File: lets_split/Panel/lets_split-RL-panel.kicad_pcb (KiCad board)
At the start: 2 copper layers, 229 x 78 mm, 116 parts, among them J2 CONN_01X04, SW1 SW_PUSH, SW10 SW_PUSH, SW11 SW_PUSH, SW12 SW_PUSH, SW13 SW_PUSH, SW14 SW_PUSH, SW15 SW_PUSH, SW16 SW_PUSH, SW17 SW_PUSH, SW18 SW_PUSH, SW19 SW_PUSH, SW2 SW_PUSH, SW20 SW_PUSH, SW21 SW_PUSH, SW22 SW_PUSH, SW23 SW_PUSH, SW24 SW_PUSH, SW3 SW_PUSH, SW4 SW_PUSH, SW5 SW_PUSH, SW6 SW_PUSH, SW7 SW_PUSH, SW8 SW_PUSH, SW9 SW_PUSH, U1 ArduinoProMicro

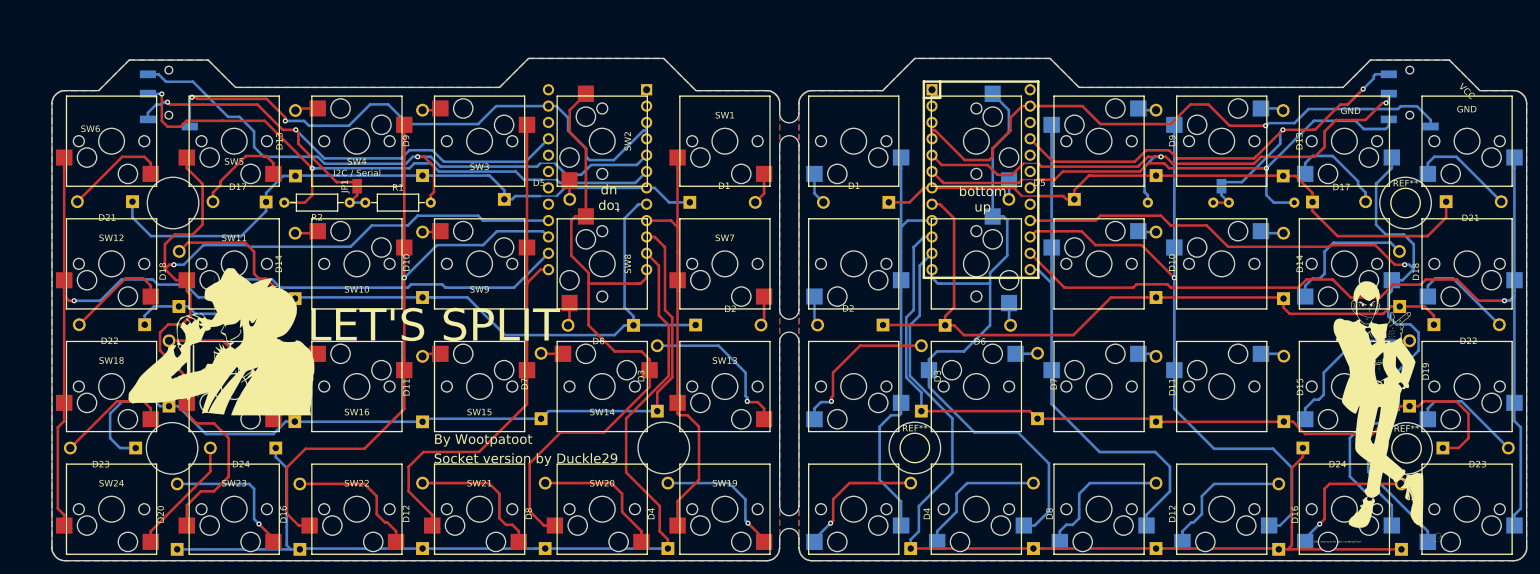
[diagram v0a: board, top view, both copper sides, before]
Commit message: Finished and panelized V3
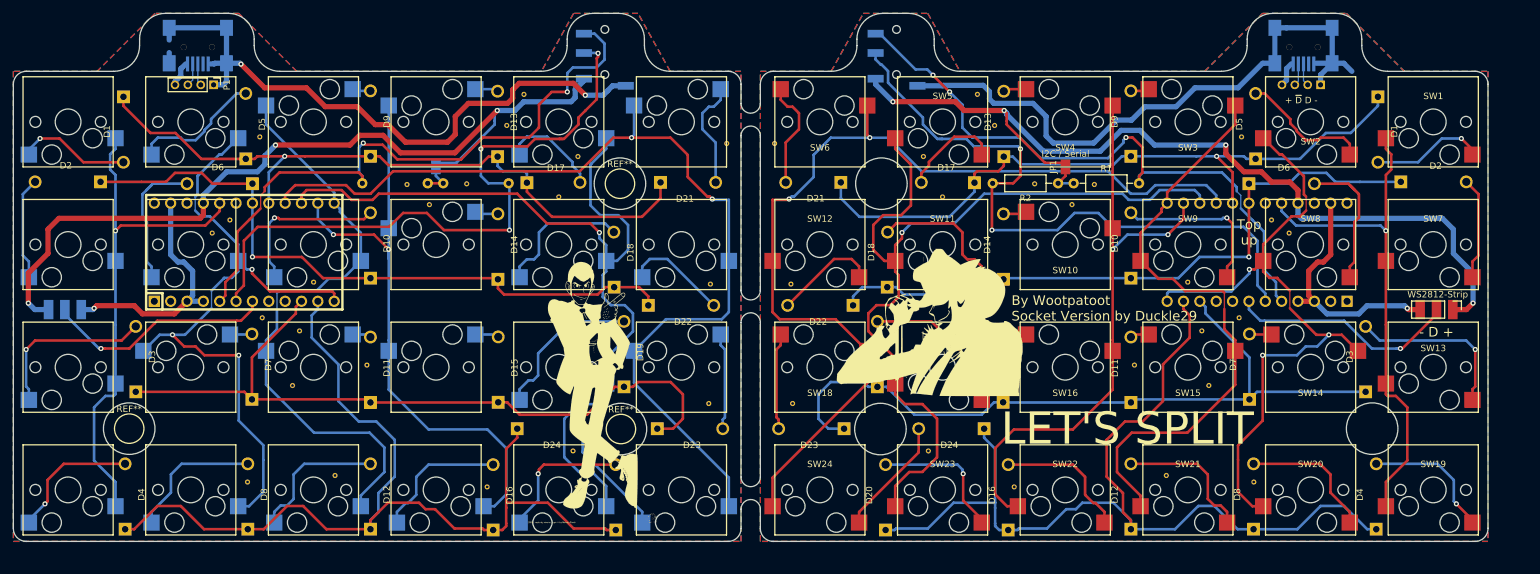
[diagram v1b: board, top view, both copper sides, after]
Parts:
- removed the D1 at (163.9, 81.3)
- removed the D1 at (133.1, 81.3)
- removed the D10 at (205.5, 96.1)
- removed the D10 at (91.5, 96.1)
- removed the D11 at (205.5, 115.4)
- removed the D11 at (91.5, 115.4)
- removed the D12 at (205.5, 135.1)
- removed the D12 at (91.5, 135.1)
- removed the D13 at (225.2, 77.2)
- removed the D13 at (71.8, 77.2)
- removed the D14 at (225.2, 96.3)
- removed the D14 at (71.8, 96.3)
- removed the D15 at (225.3, 115.4)
- removed the D15 at (71.7, 115.4)
- removed the D16 at (224.5, 135.2)
- removed the D16 at (72.5, 135.2)
- removed the D17 at (229.8, 81.3)
- removed the D17 at (67.2, 81.3)
- removed the D18 at (243.3, 97.5)
- removed the D18 at (53.7, 97.5)
- removed the D19 at (244.8, 113.0)
- removed the D19 at (52.2, 113.0)
- removed the D2 at (163.1, 100.4)
- removed the D2 at (133.9, 100.4)
- removed the D20 at (243.6, 135.2)
- removed the D20 at (53.4, 135.2)
- removed the D21 at (248.9, 81.2)
- removed the D21 at (48.1, 81.2)
- removed the D22 at (248.6, 100.3)
- removed the D22 at (48.4, 100.3)
- removed the D23 at (250.0, 119.5)
- removed the D23 at (47.0, 119.5)
- removed the D24 at (228.2, 119.5)
- removed the D24 at (68.8, 119.5)
- removed the D3 at (169.0, 113.8)
- removed the D3 at (128.0, 113.8)
- removed the D4 at (167.4, 135.1)
- removed the D4 at (129.6, 135.1)
- removed the D5 at (192.8, 80.9)
- removed the D5 at (104.2, 80.9)
- removed the D6 at (172.7, 100.5)
- removed the D6 at (124.3, 100.5)
- removed the D7 at (187.1, 115.0)
- removed the D7 at (110.0, 115.0)
- removed the D8 at (186.4, 135.1)
- removed the D8 at (110.6, 135.1)
- removed the D9 at (205.5, 77.2)
- removed the D9 at (91.5, 77.2)
- removed the G*** at (240.0, 112.8)
- removed the G*** at (231.8, 103.0)
- removed the G*** at (65.2, 103.0)
- removed the G*** at (57.0, 112.8)
- removed the J2 at (244.9, 64.3)
- removed the J2 at (52.1, 64.3)
- removed the JP1 at (215.6, 78.8)
- removed the JP1 at (81.4, 78.8)
- removed the R1 at (214.3, 81.4)
- removed the R1 at (82.7, 81.4)
- removed the R2 at (216.8, 81.4)
- removed the R2 at (80.2, 81.4)
- removed the REF** at (168.0, 119.5)
- removed the REF** at (244.3, 119.5)
- removed the REF** at (244.2, 81.5)
- removed the REF** at (52.8, 81.5)
- removed the REF** at (52.6, 119.5)
- removed the REF** at (129.0, 119.5)
- removed the SW1 at (158.5, 71.8)
- removed the SW1 at (138.5, 71.8)
- removed the SW10 at (215.7, 90.9)
- removed the SW10 at (81.3, 90.9)
- removed the SW11 at (234.7, 90.9)
- removed the SW11 at (62.3, 90.9)
- removed the SW12 at (253.8, 90.9)
- removed the SW12 at (43.2, 90.9)
- removed the SW13 at (158.5, 110.0)
- removed the SW13 at (138.5, 110.0)
- removed the SW14 at (177.6, 110.0)
- removed the SW14 at (119.5, 110.0)
- removed the SW15 at (196.6, 110.0)
- removed the SW15 at (100.4, 110.0)
- removed the SW16 at (215.7, 110.0)
- removed the SW16 at (81.3, 110.0)
- removed the SW17 at (234.7, 110.0)
- removed the SW17 at (62.3, 110.0)
- removed the SW18 at (253.8, 110.0)
- removed the SW18 at (43.2, 110.0)
- removed the SW19 at (158.5, 129.0)
- removed the SW19 at (138.5, 129.0)
- removed the SW2 at (177.6, 71.8)
- removed the SW2 at (119.5, 71.8)
- removed the SW20 at (177.6, 129.0)
- removed the SW20 at (119.5, 129.0)
- removed the SW21 at (196.6, 129.0)
- removed the SW21 at (100.4, 129.0)
- removed the SW22 at (215.7, 129.0)
- removed the SW22 at (81.3, 129.0)
- removed the SW23 at (234.7, 129.0)
- removed the SW23 at (62.3, 129.0)
- removed the SW24 at (253.8, 129.0)
- removed the SW24 at (43.2, 129.0)
- removed the SW3 at (196.6, 71.8)
- removed the SW3 at (100.4, 71.8)
- removed the SW4 at (215.7, 71.8)
- removed the SW4 at (81.3, 71.8)
- removed the SW5 at (234.7, 71.8)
- removed the SW5 at (62.3, 71.8)
- removed the SW6 at (253.8, 71.8)
- removed the SW6 at (43.2, 71.8)
- removed the SW7 at (158.5, 90.9)
- removed the SW7 at (138.5, 90.9)
- removed the SW8 at (177.6, 90.9)
- removed the SW8 at (119.5, 90.9)
- removed the SW9 at (196.6, 90.9)
- removed the SW9 at (100.4, 90.9)
- removed the U1 at (178.3, 77.8)
- removed the U1 at (118.7, 77.8)
- added D1: D, Diodes_ThroughHole:Diode_DO-41_SOD81_Horizontal_RM10, B.Cu at (239.9, 65.0)
- added D1: D, Diodes_ThroughHole:Diode_DO-41_SOD81_Horizontal_RM10, F.Cu at (45.1, 65.0)
- added D10: D, Diodes_ThroughHole:Diode_DO-41_SOD81_Horizontal_RM10, B.Cu at (201.5, 93.1)
- added D10: D, Diodes_ThroughHole:Diode_DO-41_SOD81_Horizontal_RM10, F.Cu at (83.5, 93.1)
- added D11: D, Diodes_ThroughHole:Diode_DO-41_SOD81_Horizontal_RM10, B.Cu at (201.5, 112.4)
- added D11: D, Diodes_ThroughHole:Diode_DO-41_SOD81_Horizontal_RM10, F.Cu at (83.5, 112.4)
- added D12: D, Diodes_ThroughHole:Diode_DO-41_SOD81_Horizontal_RM10, B.Cu at (201.5, 132.1)
- added D12: D, Diodes_ThroughHole:Diode_DO-41_SOD81_Horizontal_RM10, F.Cu at (83.5, 132.1)
- added D13: D, Diodes_ThroughHole:Diode_DO-41_SOD81_Horizontal_RM10, B.Cu at (181.8, 74.2)
- added D13: D, Diodes_ThroughHole:Diode_DO-41_SOD81_Horizontal_RM10, F.Cu at (103.2, 74.2)
- added D14: D, Diodes_ThroughHole:Diode_DO-41_SOD81_Horizontal_RM10, B.Cu at (181.8, 93.3)
- added D14: D, Diodes_ThroughHole:Diode_DO-41_SOD81_Horizontal_RM10, F.Cu at (103.2, 93.3)
- added D15: D, Diodes_ThroughHole:Diode_DO-41_SOD81_Horizontal_RM10, B.Cu at (181.7, 112.4)
- added D15: D, Diodes_ThroughHole:Diode_DO-41_SOD81_Horizontal_RM10, F.Cu at (103.3, 112.4)
- added D16: D, Diodes_ThroughHole:Diode_DO-41_SOD81_Horizontal_RM10, B.Cu at (182.5, 132.2)
- added D16: D, Diodes_ThroughHole:Diode_DO-41_SOD81_Horizontal_RM10, F.Cu at (102.5, 132.2)
- added D17: D, Diodes_ThroughHole:Diode_DO-41_SOD81_Horizontal_RM10, B.Cu at (177.2, 78.3)
- added D17: D, Diodes_ThroughHole:Diode_DO-41_SOD81_Horizontal_RM10, F.Cu at (107.8, 78.3)
- added D18: D, Diodes_ThroughHole:Diode_DO-41_SOD81_Horizontal_RM10, B.Cu at (163.7, 94.5)
- added D18: D, Diodes_ThroughHole:Diode_DO-41_SOD81_Horizontal_RM10, F.Cu at (121.3, 94.5)
- added D19: D, Diodes_ThroughHole:Diode_DO-41_SOD81_Horizontal_RM10, B.Cu at (162.2, 110.0)
- added D19: D, Diodes_ThroughHole:Diode_DO-41_SOD81_Horizontal_RM10, F.Cu at (122.8, 110.0)
- added D2: D, Diodes_ThroughHole:Diode_DO-41_SOD81_Horizontal_RM10, B.Cu at (243.5, 78.2)
- added D2: D, Diodes_ThroughHole:Diode_DO-41_SOD81_Horizontal_RM10, F.Cu at (41.5, 78.2)
- added D20: D, Diodes_ThroughHole:Diode_DO-41_SOD81_Horizontal_RM10, B.Cu at (163.4, 132.2)
- added D20: D, Diodes_ThroughHole:Diode_DO-41_SOD81_Horizontal_RM10, F.Cu at (121.6, 132.2)
- added D21: D, Diodes_ThroughHole:Diode_DO-41_SOD81_Horizontal_RM10, B.Cu at (158.1, 78.2)
- added D21: D, Diodes_ThroughHole:Diode_DO-41_SOD81_Horizontal_RM10, F.Cu at (126.9, 78.2)
- added D22: D, Diodes_ThroughHole:Diode_DO-41_SOD81_Horizontal_RM10, B.Cu at (158.4, 97.3)
- added D22: D, Diodes_ThroughHole:Diode_DO-41_SOD81_Horizontal_RM10, F.Cu at (126.6, 97.3)
- added D23: D, Diodes_ThroughHole:Diode_DO-41_SOD81_Horizontal_RM10, B.Cu at (157.0, 116.5)
- added D23: D, Diodes_ThroughHole:Diode_DO-41_SOD81_Horizontal_RM10, F.Cu at (128.0, 116.5)
- added D24: D, Diodes_ThroughHole:Diode_DO-41_SOD81_Horizontal_RM10, B.Cu at (178.8, 116.5)
- added D24: D, Diodes_ThroughHole:Diode_DO-41_SOD81_Horizontal_RM10, F.Cu at (106.2, 116.5)
- added D3: D, Diodes_ThroughHole:Diode_DO-41_SOD81_Horizontal_RM10, B.Cu at (238.0, 110.8)
- added D3: D, Diodes_ThroughHole:Diode_DO-41_SOD81_Horizontal_RM10, F.Cu at (47.0, 110.8)
- added D4: D, Diodes_ThroughHole:Diode_DO-41_SOD81_Horizontal_RM10, B.Cu at (239.6, 132.1)
- added D4: D, Diodes_ThroughHole:Diode_DO-41_SOD81_Horizontal_RM10, F.Cu at (45.4, 132.1)
- added D5: D, Diodes_ThroughHole:Diode_DO-41_SOD81_Horizontal_RM10, B.Cu at (220.9, 74.6)
- added D5: D, Diodes_ThroughHole:Diode_DO-41_SOD81_Horizontal_RM10, F.Cu at (64.1, 74.6)
- added D6: D, Diodes_ThroughHole:Diode_DO-41_SOD81_Horizontal_RM10, B.Cu at (219.9, 78.4)
- added D6: D, Diodes_ThroughHole:Diode_DO-41_SOD81_Horizontal_RM10, F.Cu at (65.1, 78.4)
- added D7: D, Diodes_ThroughHole:Diode_DO-41_SOD81_Horizontal_RM10, B.Cu at (219.9, 112.0)
- added D7: D, Diodes_ThroughHole:Diode_DO-41_SOD81_Horizontal_RM10, F.Cu at (65.0, 112.0)
- added D8: D, Diodes_ThroughHole:Diode_DO-41_SOD81_Horizontal_RM10, B.Cu at (220.6, 132.1)
- added D8: D, Diodes_ThroughHole:Diode_DO-41_SOD81_Horizontal_RM10, F.Cu at (64.4, 132.1)
- added D9: D, Diodes_ThroughHole:Diode_DO-41_SOD81_Horizontal_RM10, B.Cu at (201.5, 74.2)
- added D9: D, Diodes_ThroughHole:Diode_DO-41_SOD81_Horizontal_RM10, F.Cu at (83.5, 74.2)
- added G***: LOGO, LOGO, B.Cu at (167.0, 109.8)
- added G***: LOGO, LOGO, F.Cu at (175.2, 100.0)
- added G***: LOGO, LOGO, B.Cu at (109.8, 100.0)
- added G***: LOGO, LOGO, F.Cu at (118.0, 109.8)
- added J2: CONN_01X04, Connectors:4ucon-20153, B.Cu at (165.1, 58.0)
- added J2: CONN_01X04, Connectors:4ucon-20153, B.Cu at (119.9, 58.0)
- added JP1: I2C / Serial, Jumpers:Solder-jumper-NO, F.Cu at (191.4, 75.8)
- added JP1: I2C / Serial, Jumpers:Solder-jumper-NO, B.Cu at (93.6, 75.8)
- added P1: USB-rewire, Pin_Headers:Pin_Header_Straight_1x04_Pitch2.00mm, B.Cu at (231.0, 63.1)
- added P1: USB-rewire, Pin_Headers:Pin_Header_Straight_1x04_Pitch2.00mm, F.Cu at (59.1, 63.1)
- added P2: USB_OTG, Connectors:USB-Mini-B-SMD, B.Cu at (228.3, 56.0)
- added P2: USB_OTG, Connectors:USB-Mini-B-SMD, B.Cu at (56.6, 56.0)
- added P3: WS2812-Strip, SMD_PAD_1x03_Pitch2.54mm, F.Cu at (251.5, 98.0)
- added P3: WS2812-Strip, SMD_PAD_1x03_Pitch2.54mm, B.Cu at (33.5, 98.0)
- added R1: 4k7, Resistors_ThroughHole:R_Axial_DIN0207_L6.3mm_D2.5mm_P10.16mm_Horizontal, F.Cu at (192.7, 78.4)
- added R1: 4k7, Resistors_ThroughHole:R_Axial_DIN0207_L6.3mm_D2.5mm_P10.16mm_Horizontal, B.Cu at (92.3, 78.4)
- added R2: 4k7, Resistors_ThroughHole:R_Axial_DIN0207_L6.3mm_D2.5mm_P10.16mm_Horizontal, F.Cu at (190.2, 78.4)
- added R2: 4k7, Resistors_ThroughHole:R_Axial_DIN0207_L6.3mm_D2.5mm_P10.16mm_Horizontal, B.Cu at (94.8, 78.4)
- added REF**: 1pin, Connect:1pin, B.Cu at (239.0, 116.5)
- added REF**: 1pin, Connect:1pin, B.Cu at (170.1, 120.0)
- added REF**: 1pin, Connect:1pin, B.Cu at (149.0, 112.6)
- added REF**: 1pin, Connect:1pin, B.Cu at (148.8, 94.0)
- added REF**: 1pin, Connect:1pin, B.Cu at (146.2, 72.2)
- added REF**: 1pin, Connect:1pin, B.Cu at (180.4, 69.4)
- added REF**: 1pin, Connect:1pin, B.Cu at (169.3, 74.2)
- added REF**: 1pin, Connect:1pin, B.Cu at (218.7, 71.2)
- added REF**: 1pin, Connect:1pin, B.Cu at (212.6, 101.3)
- added REF**: 1pin, Connect:1pin, B.Cu at (218.3, 99.3)
- added REF**: 1pin, Connect:1pin, B.Cu at (226.1, 86.1)
- added REF**: 1pin, Connect:1pin, B.Cu at (162.7, 116.5)
- added REF**: 1pin, Connect:1pin, B.Cu at (223.4, 84.1)
- added REF**: 1pin, Connect:1pin, B.Cu at (210.4, 93.7)
- added REF**: 1pin, Connect:1pin, B.Cu at (172.3, 80.5)
- added REF**: 1pin, Connect:1pin, B.Cu at (192.4, 81.7)
- added REF**: 1pin, Connect:1pin, B.Cu at (195.9, 78.6)
- added REF**: 1pin, Connect:1pin, B.Cu at (186.6, 78.5)
- added REF**: 1pin, Connect:1pin, F.Cu at (98.4, 78.5)
- added REF**: 1pin, Connect:1pin, F.Cu at (89.1, 78.6)
- added REF**: 1pin, Connect:1pin, F.Cu at (92.6, 81.7)
- added REF**: 1pin, Connect:1pin, F.Cu at (112.7, 80.5)
- added REF**: 1pin, Connect:1pin, B.Cu at (162.8, 78.5)
- added REF**: 1pin, Connect:1pin, F.Cu at (74.6, 93.7)
- added REF**: 1pin, Connect:1pin, F.Cu at (61.6, 84.1)
- added REF**: 1pin, Connect:1pin, F.Cu at (58.9, 86.1)
- added REF**: 1pin, Connect:1pin, F.Cu at (66.7, 99.3)
- added REF**: 1pin, Connect:1pin, F.Cu at (72.4, 101.3)
- added REF**: 1pin, Connect:1pin, F.Cu at (66.3, 71.2)
- added REF**: 1pin, Connect:1pin, F.Cu at (115.7, 74.2)
- added REF**: 1pin, Connect:1pin, F.Cu at (104.6, 69.4)
- added REF**: 1pin, Connect:1pin, F.Cu at (138.8, 72.2)
- added REF**: 1pin, Connect:1pin, F.Cu at (136.2, 94.0)
- added REF**: 1pin, Connect:1pin, B.Cu at (177.7, 64.6)
- added REF**: 1pin, Connect:1pin, F.Cu at (136.0, 112.6)
- added REF**: 1pin, Connect:1pin, F.Cu at (114.9, 120.0)
- added REF**: 1pin, Connect:1pin, F.Cu at (101.6, 125.5)
- added REF**: 1pin, Connect:1pin, F.Cu at (64.4, 124.8)
- added REF**: 1pin, Connect:1pin, F.Cu at (78.0, 123.8)
- added REF**: 1pin, Connect:1pin, F.Cu at (71.3, 109.8)
- added REF**: 1pin, Connect:1pin, F.Cu at (82.9, 106.6)
- added REF**: 1pin, Connect:1pin, F.Cu at (107.3, 64.6)
- added REF**: 1pin, Connect:1pin, F.Cu at (122.2, 78.5)
- added REF**: 1pin, Connect:1pin, F.Cu at (122.3, 116.5)
- added REF**: 1pin, Connect:1pin, B.Cu at (202.1, 106.6)
- added REF**: 1pin, Connect:1pin, F.Cu at (46.0, 116.5)
- added REF**: 1pin, Connect:1pin, B.Cu at (213.7, 109.8)
- added REF**: 1pin, Connect:1pin, B.Cu at (207.0, 123.8)
- added REF**: 1pin, Connect:1pin, B.Cu at (220.6, 124.8)
- added REF**: 1pin, Connect:1pin, B.Cu at (183.4, 125.5)
- added SW1: SW_PUSH, CherryMX:Kailh-socket, B.Cu at (248.5, 68.8)
- added SW1: SW_PUSH, CherryMX:Kailh-socket, F.Cu at (36.5, 68.8)
- added SW10: SW_PUSH, CherryMX:Kailh-socket, B.Cu at (191.3, 87.9)
- added SW10: SW_PUSH, CherryMX:Kailh-socket, F.Cu at (93.7, 87.9)
- added SW11: SW_PUSH, CherryMX:Kailh-socket, B.Cu at (172.3, 87.9)
- added SW11: SW_PUSH, CherryMX:Kailh-socket, F.Cu at (112.7, 87.9)
- added SW12: SW_PUSH, CherryMX:Kailh-socket, B.Cu at (153.2, 87.9)
- added SW12: SW_PUSH, CherryMX:Kailh-socket, F.Cu at (131.8, 87.9)
- added SW13: SW_PUSH, CherryMX:Kailh-socket, B.Cu at (248.5, 107.0)
- added SW13: SW_PUSH, CherryMX:Kailh-socket, F.Cu at (36.5, 107.0)
- added SW14: SW_PUSH, CherryMX:Kailh-socket, B.Cu at (229.4, 107.0)
- added SW14: SW_PUSH, CherryMX:Kailh-socket, F.Cu at (55.5, 107.0)
- added SW15: SW_PUSH, CherryMX:Kailh-socket, B.Cu at (210.4, 107.0)
- added SW15: SW_PUSH, CherryMX:Kailh-socket, F.Cu at (74.6, 107.0)
- added SW16: SW_PUSH, CherryMX:Kailh-socket, B.Cu at (191.3, 107.0)
- added SW16: SW_PUSH, CherryMX:Kailh-socket, F.Cu at (93.7, 107.0)
- added SW17: SW_PUSH, CherryMX:Kailh-socket, B.Cu at (172.3, 107.0)
- added SW17: SW_PUSH, CherryMX:Kailh-socket, F.Cu at (112.7, 107.0)
- added SW18: SW_PUSH, CherryMX:Kailh-socket, B.Cu at (153.2, 107.0)
- added SW18: SW_PUSH, CherryMX:Kailh-socket, F.Cu at (131.8, 107.0)
- added SW19: SW_PUSH, CherryMX:Kailh-socket, B.Cu at (248.5, 126.0)
- added SW19: SW_PUSH, CherryMX:Kailh-socket, F.Cu at (36.5, 126.0)
- added SW2: SW_PUSH, CherryMX:Kailh-socket, B.Cu at (229.4, 68.8)
- added SW2: SW_PUSH, CherryMX:Kailh-socket, F.Cu at (55.5, 68.8)
- added SW20: SW_PUSH, CherryMX:Kailh-socket, B.Cu at (229.4, 126.0)
- added SW20: SW_PUSH, CherryMX:Kailh-socket, F.Cu at (55.5, 126.0)
- added SW21: SW_PUSH, CherryMX:Kailh-socket, B.Cu at (210.4, 126.0)
- added SW21: SW_PUSH, CherryMX:Kailh-socket, F.Cu at (74.6, 126.0)
- added SW22: SW_PUSH, CherryMX:Kailh-socket, B.Cu at (191.3, 126.0)
- added SW22: SW_PUSH, CherryMX:Kailh-socket, F.Cu at (93.7, 126.0)
- added SW23: SW_PUSH, CherryMX:Kailh-socket, B.Cu at (172.3, 126.0)
- added SW23: SW_PUSH, CherryMX:Kailh-socket, F.Cu at (112.7, 126.0)
- added SW24: SW_PUSH, CherryMX:Kailh-socket, B.Cu at (153.2, 126.0)
- added SW24: SW_PUSH, CherryMX:Kailh-socket, F.Cu at (131.8, 126.0)
- added SW3: SW_PUSH, CherryMX:Kailh-socket, B.Cu at (210.4, 68.8)
- added SW3: SW_PUSH, CherryMX:Kailh-socket, F.Cu at (74.6, 68.8)
- added SW4: SW_PUSH, CherryMX:Kailh-socket, B.Cu at (191.3, 68.8)
- added SW4: SW_PUSH, CherryMX:Kailh-socket, F.Cu at (93.7, 68.8)
- added SW5: SW_PUSH, CherryMX:Kailh-socket, B.Cu at (172.3, 68.8)
- added SW5: SW_PUSH, CherryMX:Kailh-socket, F.Cu at (112.7, 68.8)
- added SW6: SW_PUSH, Kailh-socket, B.Cu at (153.2, 68.8)
- added SW6: SW_PUSH, Kailh-socket, F.Cu at (131.8, 68.8)
- added SW7: SW_PUSH, CherryMX:Kailh-socket, B.Cu at (248.5, 87.9)
- added SW7: SW_PUSH, CherryMX:Kailh-socket, F.Cu at (36.5, 87.9)
- added SW8: SW_PUSH, CherryMX:Kailh-socket, B.Cu at (229.4, 87.9)
- added SW8: SW_PUSH, CherryMX:Kailh-socket, F.Cu at (55.5, 87.9)
- added SW9: SW_PUSH, CherryMX:Kailh-socket, B.Cu at (210.4, 87.9)
- added SW9: SW_PUSH, CherryMX:Kailh-socket, F.Cu at (74.6, 87.9)
- added U1: ArduinoProMicro, plug-in-modules:ArduinoProMicro, B.Cu at (221.1, 89.1)
- added U1: ArduinoProMicro, plug-in-modules:ArduinoProMicro, F.Cu at (63.9, 89.1)
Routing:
- net VCC: track 162.2 -> 264.9 mm, vias 4 -> 7
- net GND: track 187.7 -> 274.0 mm, vias 3 -> 4
- net Net-(P3-Pad2): track 0.00 -> 71.7 mm, vias 0 -> 2
- net Net-(D10-Pad2): track 5.64 -> 50.6 mm, vias 0 -> 2
- net Net-(D6-Pad2): track 7.11 -> 44.3 mm
- net Net-(D5-Pad2): track 5.91 -> 40.8 mm
- net col0: track 131.8 -> 160.1 mm, vias 0 -> 2
- net Net-(D1-Pad2): track 9.99 -> 35.4 mm, vias 0 -> 2
- net col2: track 162.1 -> 186.7 mm
- net row2: track 256.4 -> 232.4 mm
- net row1: track 229.7 -> 206.8 mm, vias 0 -> 2
- net Net-(D2-Pad2): track 9.24 -> 32.0 mm
- net col5: track 280.7 -> 302.0 mm, vias 2 -> 4
- net SCL/D3: track 183.8 -> 203.9 mm, vias 3 -> 5
- net col3: track 206.7 -> 188.9 mm, vias 2 -> 4
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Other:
- board size 229 x 78 mm -> 229 x 82 mm
- rule trace_min: 0.1524 -> 0.006
- board text added: "+ ~D~ D -"
- board text added: "- D +"
- board text added: "- D ~D~ +"
- board text added: "By Wootpatoot Socket Version by Duckle29"
- board text added: "Top up"
- board text removed: "By Wootpatoot"
- board text removed: "GND"
- board text removed: "Socket version by Duckle29"
- board text removed: "VCC"
- board text removed: "top up"

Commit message: Changed to actually aquireable TRRS connector
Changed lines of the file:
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@@
 (kicad_pcb (version 4) (host pcbnew 4.0.1-stable)
   (general
-    (links 0)
-    (no_connects 7)
-    (area 27.924999 51.924999 257.075001 134.075001)
+    (links 285)
+    (no_connects 55)
+    (area 27.924999 49.747599 257.075001 134.075001)
     (thickness 1.6)
-    (drawings 72)
+    (drawings 74)
     (tracks 1221)
     (zones 0)
@@
   )
   (setup
-    (last_trace_width 0.8128)
+    (last_trace_width 0.1524)
     (user_trace_width 0.2032)
     (user_trace_width 0.4064)
@@
       (net 36 col5))
   )
+  (dimension 82 (width 0.3) (layer Cmts.User)
+    (gr_text "82,000 mm" (at 263.35 93 90) (layer Cmts.User)
+      (effects (font (size 1.5 1.5) (thickness 0.3)))
+    )
+    (feature1 (pts (xy 257 52) (xy 264.7 52)))
+    (feature2 (pts (xy 257 134) (xy 264.7 134)))
+    (crossbar (pts (xy 262 134) (xy 262 52)))
+    (arrow1a (pts (xy 262 52) (xy 262.586421 53.126504)))
+    (arrow1b (pts (xy 262 52) (xy 261.413579 53.126504)))
+    (arrow2a (pts (xy 262 134) (xy 262.586421 132.873496)))
+    (arrow2b (pts (xy 262 134) (xy 261.413579 132.873496)))
+  )
+  (dimension 229 (width 0.3) (layer Cmts.User)
+    (gr_text "229,000 mm" (at 142.5 139.35) (layer Cmts.User)
+      (effects (font (size 1.5 1.5) (thickness 0.3)))
+    )
+    (feature1 (pts (xy 257 134) (xy 257 140.7)))
+    (feature2 (pts (xy 28 134) (xy 28 140.7)))
+    (crossbar (pts (xy 28 138) (xy 257 138)))
+    (arrow1a (pts (xy 257 138) (xy 255.873496 138.586421)))
+    (arrow1b (pts (xy 257 138) (xy 255.873496 137.413579)))
+    (arrow2a (pts (xy 28 138) (xy 29.126504 138.586421)))
+    (arrow2b (pts (xy 28 138) (xy 29.126504 137.413579)))
+  )
   (gr_line (start 141 63) (end 141 66) (layer Edge.Cuts) (width 0.15))
   (gr_line (start 144 66) (end 144 63) (layer Edge.Cuts) (width 0.15))
@@
   (gr_line (start 155 61) (end 146 61) (angle 90) (layer Edge.Cuts) (width 0.15))
   (gr_line (start 146 134) (end 255 134) (angle 90) (layer Edge.Cuts) (width 0.15))
-  (gr_text "Top\nup\n" (at 219.9 86 360) (layer F.SilkS)
+  (gr_text "Top\nup\n" (at 219.9 86) (layer F.SilkS)
     (effects (font (size 1.5 1.5) (thickness 0.3)))
   )
-  (gr_text "By Wootpatoot\nSocket Version by Duckle29" (at 183 97.8 360) (layer F.SilkS)
+  (gr_text "By Wootpatoot\nSocket Version by Duckle29" (at 183 97.8) (layer F.SilkS)
     (effects (font (size 1.5 1.5) (thickness 0.3)) (justify left))
   )
-  (gr_text "LET'S SPLIT" (at 201 116.5 360) (layer F.SilkS)
+  (gr_text "LET'S SPLIT" (at 201 116.5) (layer F.SilkS)
     (effects (font (size 5 5) (thickness 0.3)))
   )
@@
   (gr_arc (start 255 63) (end 257 63) (angle -90) (layer Edge.Cuts) (width 0.15))
   (gr_line (start 233.4 52) (end 223.6 52) (layer Edge.Cuts) (width 0.15))
-  (gr_text "- D +" (at 249 101.5 360) (layer F.SilkS)
+  (gr_text "- D +" (at 249 101.5) (layer F.SilkS)
     (effects (font (size 1.5 1.5) (thickness 0.3)))
   )
